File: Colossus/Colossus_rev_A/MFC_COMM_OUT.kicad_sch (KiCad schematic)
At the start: 16 parts, among them J5 Conn_01x01, J6 Conn_01x03, J7 Conn_01x02, Q5 2SC4213, U4 MCP6L01Rx-xOT, U6 AD9833xRM, Y2 MFC

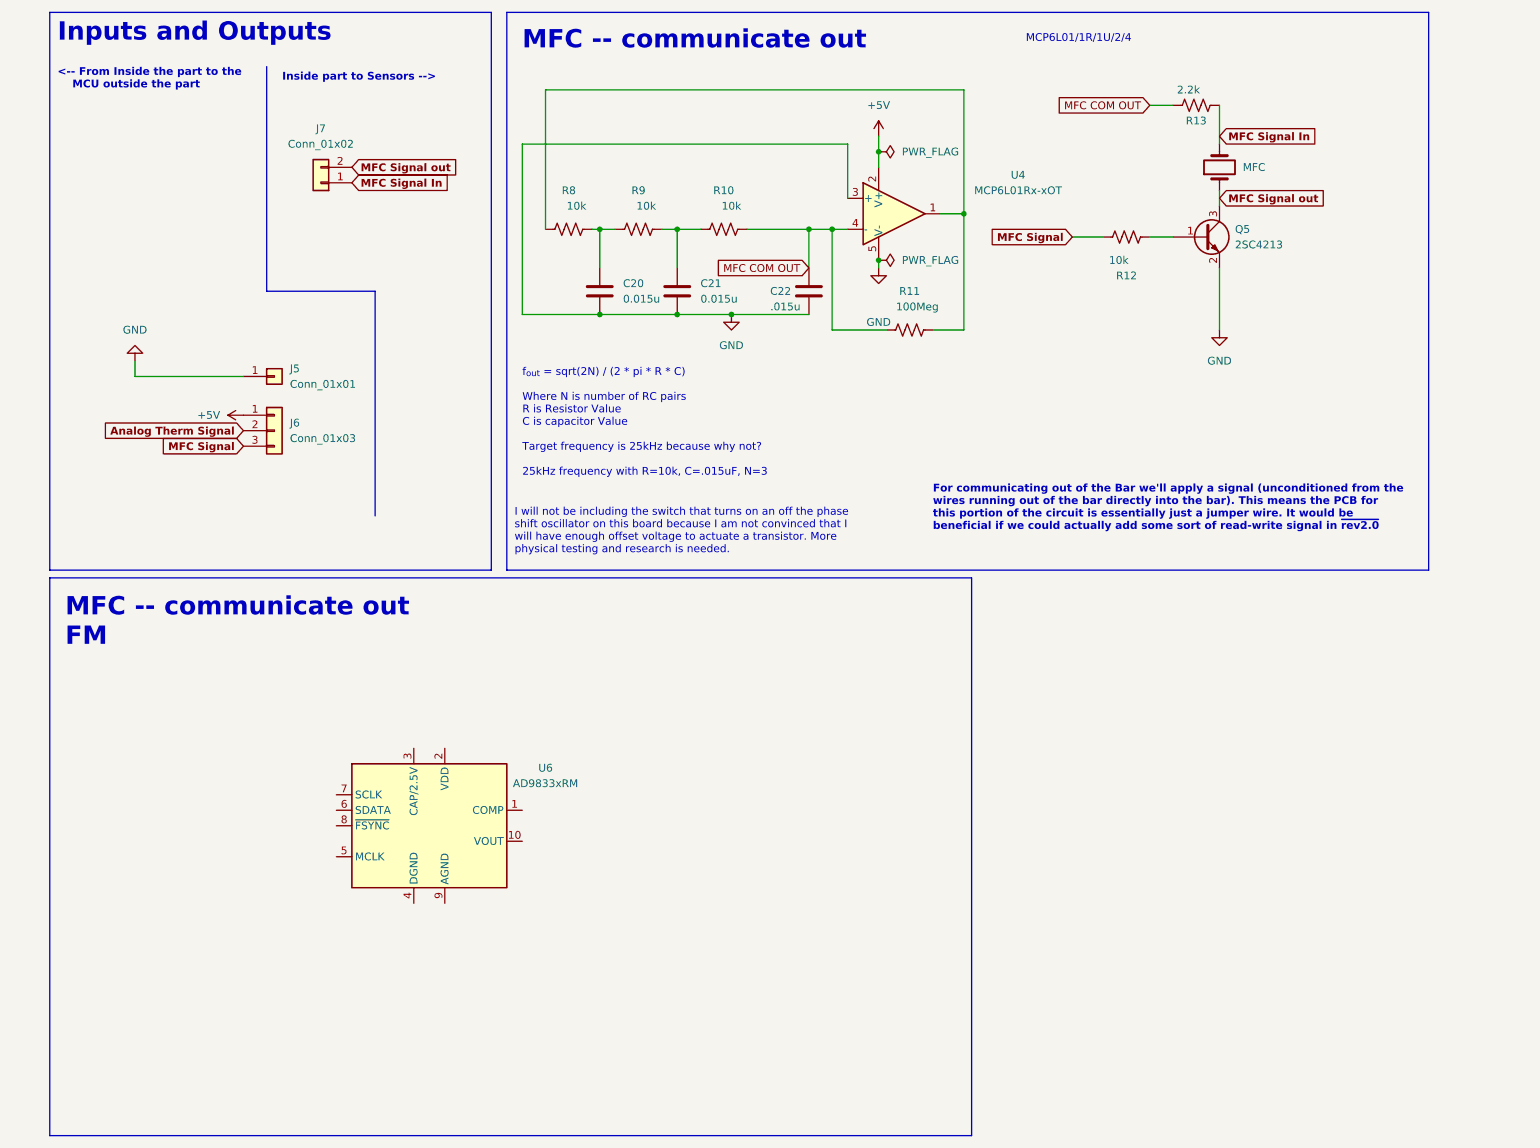
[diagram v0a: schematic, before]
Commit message: pushing to save
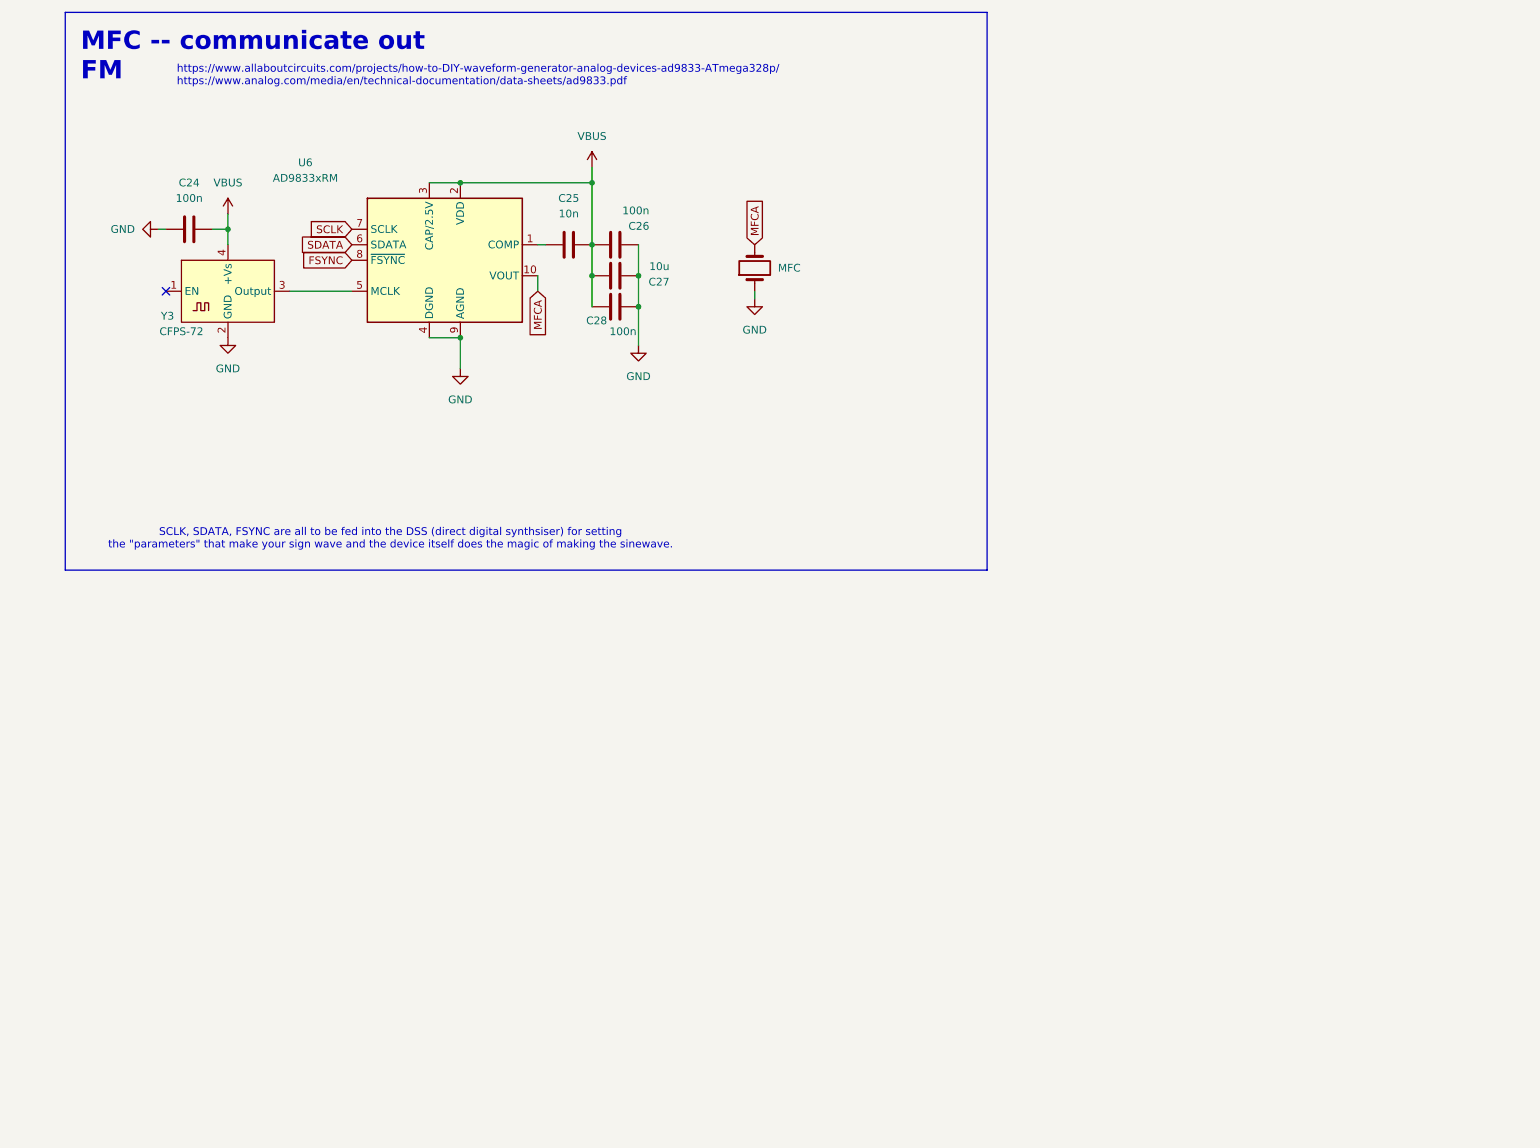
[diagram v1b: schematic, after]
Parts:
- removed C20, C21: 0.015u, Capacitor_SMD:C_0402_1005Metric, symbol Device:C
- removed C22: .015u, Capacitor_SMD:C_0402_1005Metric, symbol Device:C
- removed J5: Conn_01x01, Connector_Wire:SolderWire-0.1sqmm_1x01_D0.4mm_OD1mm, symbol Connector_Generic:Conn_01x01
- removed J6: Conn_01x03, Connector_Wire:SolderWire-0.1sqmm_1x03_P3.6mm_D0.4mm_OD1mm, symbol Connector_Generic:Conn_01x03
- removed J7: Conn_01x02, Connector_Wire:SolderWire-0.1sqmm_1x02_P3.6mm_D0.4mm_OD1mm, symbol Connector_Generic:Conn_01x02
- removed Q5: 2SC4213, Package_TO_SOT_SMD:SOT-323_SC-70, symbol Transistor_BJT:2SC4213
- removed R10, R12, R8, R9: 10k, Resistor_SMD:R_0402_1005Metric, symbol Device:R_US
- removed R11: 100Meg, Resistor_SMD:R_0402_1005Metric, symbol Device:R_US
- removed R13: 2.2k, Resistor_SMD:R_0402_1005Metric, symbol Device:R_US
- removed U4: MCP6L01Rx-xOT, Package_TO_SOT_SMD:SOT-23-5, symbol Amplifier_Operational:MCP6L01Rx-xOT
- removed Y2: MFC, Crystal:Crystal_AT310_D3.0mm_L10.0mm_Horizontal_1EP_style1, symbol Device:Crystal
- added C24, C26, C28: 100n, Capacitor_SMD:C_0201_0603Metric, symbol Device:C
- added C25: 10n, Capacitor_SMD:C_0201_0603Metric, symbol Device:C
- added C27: 10u, Capacitor_SMD:C_0201_0603Metric, symbol Device:C
- added Y3: CFPS-72, Oscillator:Oscillator_SMD_IQD_IQXO70-4Pin_7.5x5.0mm, symbol Oscillator:CFPS-72
- added Y4: MFC, Crystal:Crystal_AT310_D3.0mm_L10.0mm_Horizontal_1EP_style1, symbol Device:Crystal
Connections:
- net GND: now also U6.4 (DGND), U6.9 (AGND), C24.1, C26.1, C27.1, C28.2, Y3.2 (GND), Y4.1
- net at U6.1 (COMP): now also C25.1
- net MFCA: now reaches U6.10 (VOUT)
- net MFCA: now also Y4.2
- net VBUS: now reaches U6.2 (VDD)
- net VBUS: now also U6.3 (CAP/2.5V), C24.2, C25.2, C26.2, C27.2, C28.1, Y3.4 (+Vs)
- net at U6.5 (MCLK): now also Y3.3 (Output)
- net SDATA: now reaches U6.6 (SDATA)
- net SCLK: now reaches U6.7 (SCLK)
- net FSYNC: now reaches U6.8 (~{FSYNC})
- no-connect marks 0 -> 1
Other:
- note added: "SCLK, SDATA, FSYNC are all to be fed into the DSS (direct digital synthsiser) for setting the "parameters" that make your sign wave and the device itself does the magic of making the sinewave."
- note added: "https://www.allaboutcircuits.com/projects/how-to-DIY-waveform-generator-analog-devices-ad9833-ATmega328p/ https://www.analog.com/media/en/technical-documentation/data-sheets/ad9833.pdf"
- note removed: "<-- From Inside the part to the MCU outside the part"
- note removed: "For communicating out of the Bar we'll apply a signal (unconditioned from the wires running out of the bar directly into the bar). This means the PCB for this portion of the circuit is essentially just a jumper wire. It would be beneficial if we could actually add some sort of read-write signal in ~{rev2.0}"
- note removed: "I will not be including the switch that turns on an off the phase shift oscillator on this board because I am not convinced that I will have enough offset voltage to actuate a transistor. More physical testing and research is needed."
- note removed: "Inputs and Outputs"
- note removed: "Inside part to Sensors -->"
- note removed: "MCP6L01/1R/1U/2/4"
- note removed: "MFC -- communicate out"
- note removed: "f_{out} = sqrt(2N) / (2 * pi * R * C) Where N is number of RC pairs R is Resistor Value C is capacitor Value Target frequency is 25kHz because why not? 25kHz frequency with R=10k, C=.015uF, N=3"
- moved on the sheet: U6
